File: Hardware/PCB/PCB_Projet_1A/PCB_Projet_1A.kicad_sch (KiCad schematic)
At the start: 36 parts, among them J1 Conn_01x02, J10 Conn_ST_STDC14, J11 Conn_01x03, J12 Conn_01x03, J2 Conn_01x02, J3 Conn_01x02, J4 BU33SD5WG-TR, J5 R-78B5.0-2.0, J6 Conn_01x04, J7 Conn_01x04, J8 Conn_01x04, J9 Conn_01x04, U1 STM32L552CCTx

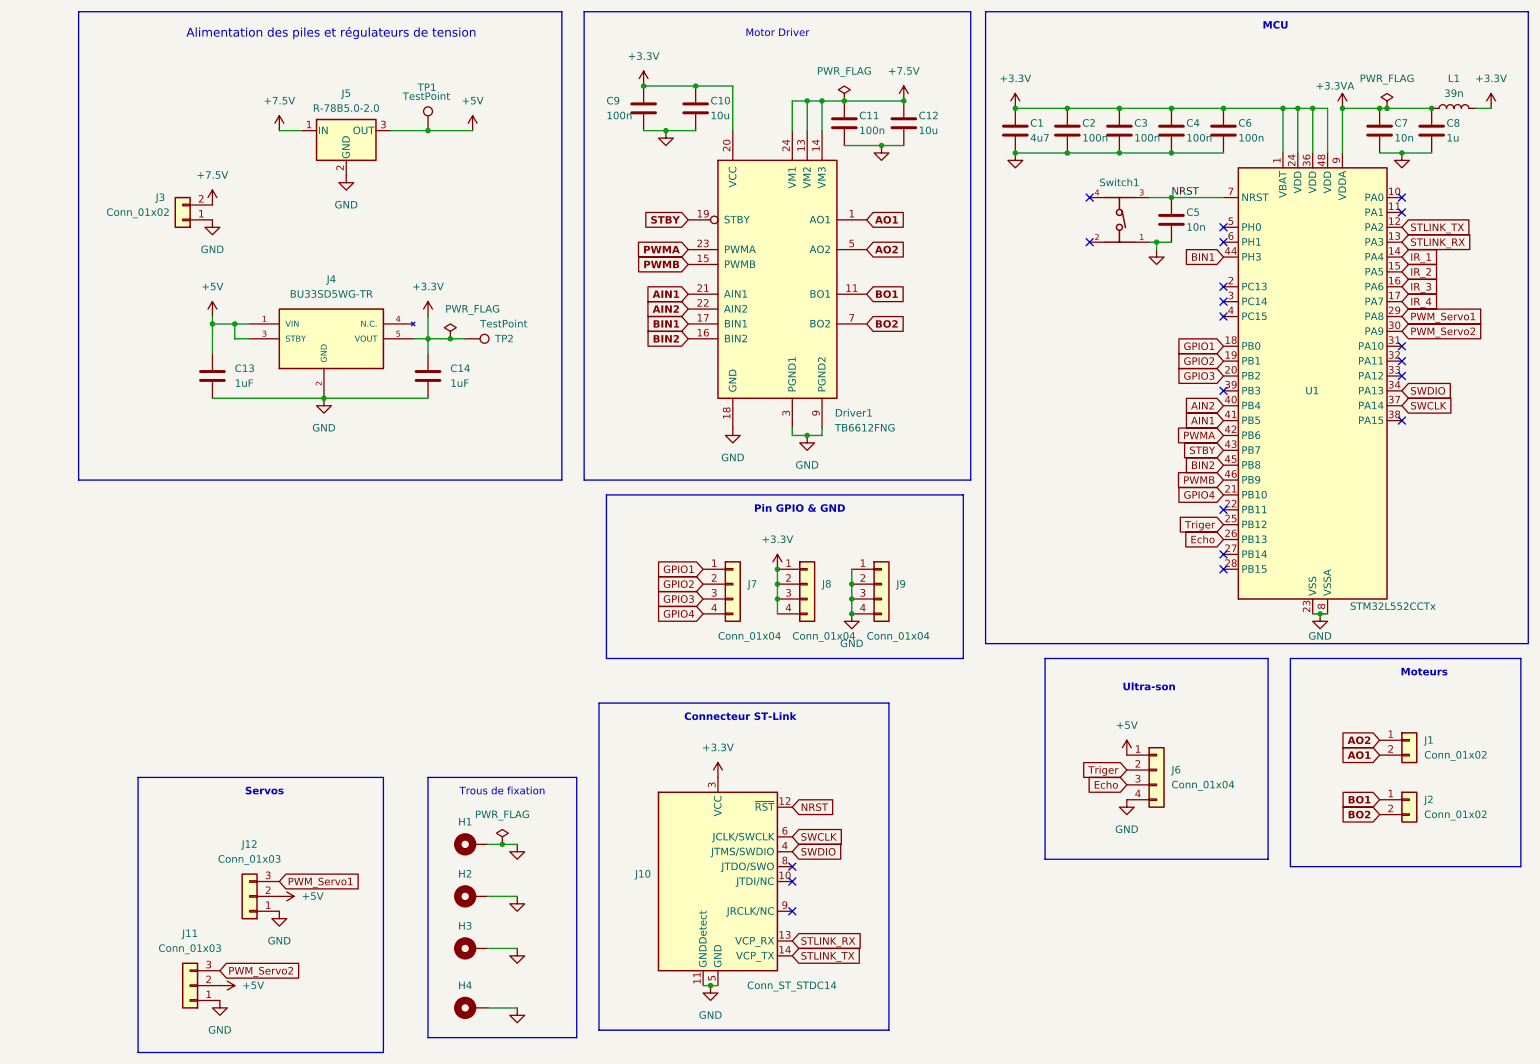
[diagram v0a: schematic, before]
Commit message: modification schematique
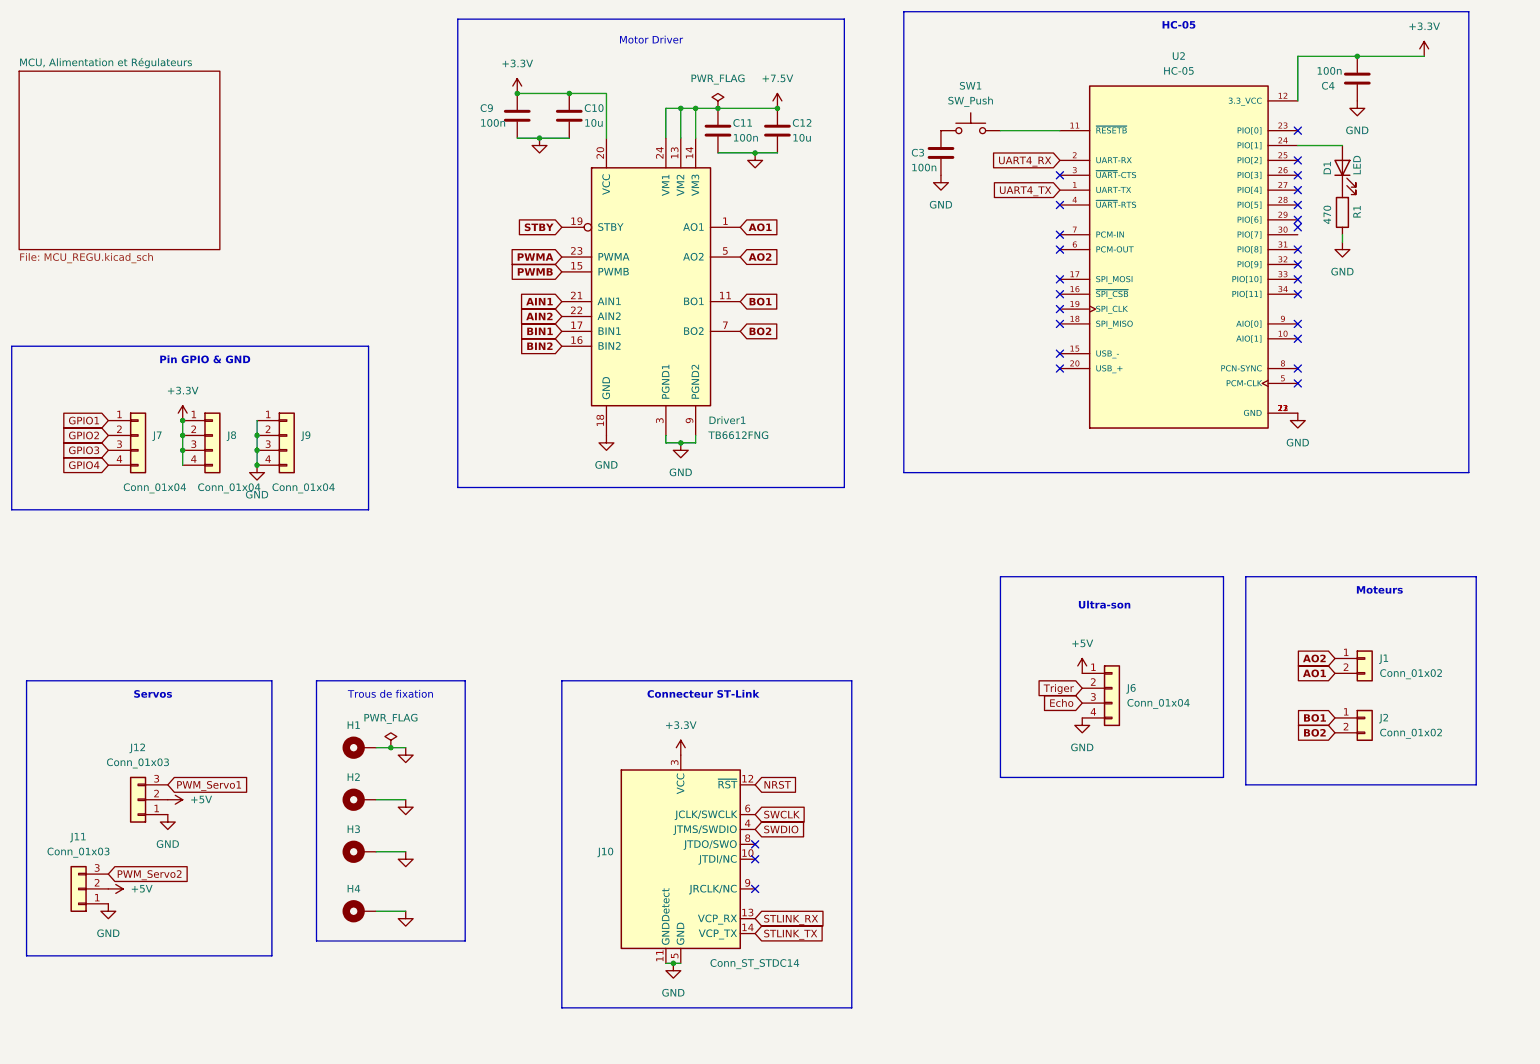
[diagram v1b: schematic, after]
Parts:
- removed C1: 4u7, Capacitor_SMD:C_0805_2012Metric, symbol Device:C
- removed C13, C14: 1uF, Capacitor_SMD:C_0603_1608Metric_Pad1.08x0.95mm_HandSolder, symbol Device:C
- removed C2, C6: 100n, Capacitor_SMD:C_0402_1005Metric, symbol Device:C
- removed C5, C7: 10n, Capacitor_SMD:C_0402_1005Metric, symbol Device:C
- removed C8: 1u, Capacitor_SMD:C_0402_1005Metric, symbol Device:C
- removed J3: Conn_01x02, Connector_JST:JST_XH_S2B-XH-A-1_1x02_P2.50mm_Horizontal, symbol Connector_Generic:Conn_01x02
- removed J4: BU33SD5WG-TR, BU33SD5WG-TR:SOT95P280X125-5N, symbol BU33SD5WG-TR:BU33SD5WG-TR
- removed J5: R-78B5.0-2.0, Converter_DCDC:Converter_DCDC_RECOM_R-78B-2.0_THT, symbol Regulator_Switching:R-78B5.0-2.0
- removed L1: 39n, Inductor_SMD:L_0603_1608Metric, symbol Device:L
- removed Switch1: 430471025826, boutonSMD_wurth430471025826:430471025826, symbol boutonSMD_wurth430471025826:430471025826
- removed TP1, TP2: TestPoint, TestPoint:TestPoint_Pad_D2.0mm, symbol Connector:TestPoint
- removed U1: STM32L552CCTx, Package_QFP:LQFP-48_7x7mm_P0.5mm, symbol MCU_ST_STM32L5:STM32L552CCTx
- added D1: LED, symbol Device:LED
- added R1: 470, symbol Device:R
- added SW1: SW_Push, symbol Switch:SW_Push
- added U2: HC-05, HC-05:XCVR_HC-05, symbol HC-05:HC-05
- C3, C4: footprint Capacitor_SMD:C_0402_1005Metric -> (none)
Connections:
- net +3.3V: now also U2.12 (3.3_VCC); no longer C3.1
- net GND: now also C3.1, R1.1, U2.13 (GND), U2.21 (GND), U2.22 (GND); no longer C3.2
- new net: SW1.2, U2.11 (~{RESETB})
- new net: D1.2 (A), U2.24 (PIO[1])
- new net: D1.1 (K), R1.2
- new net: C3.2, SW1.1
- new net UART4_RX: U2.2 (UART-RX)
- new net UART4_TX: U2.1 (UART-TX)
- no-connect marks 20 -> 28
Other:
- added sheet MCU, Alimentation et Régulateurs (MCU_REGU.kicad_sch)
- note added: "HC-05"
- note removed: "Alimentation des piles et régulateurs de tension"
- note removed: "MCU"
- moved on the sheet: C10, C11, C12, C9, Driver1, H1, H2, H3, H4, J1, J10, J11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
